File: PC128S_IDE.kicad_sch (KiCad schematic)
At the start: 15 parts, among them J1 User 2MHZ Port, J3 Conn_01x02_Male, J5 Conn_01x02_Male, P1 IDE02x20, U1 74HCT02, U2 74HCT139

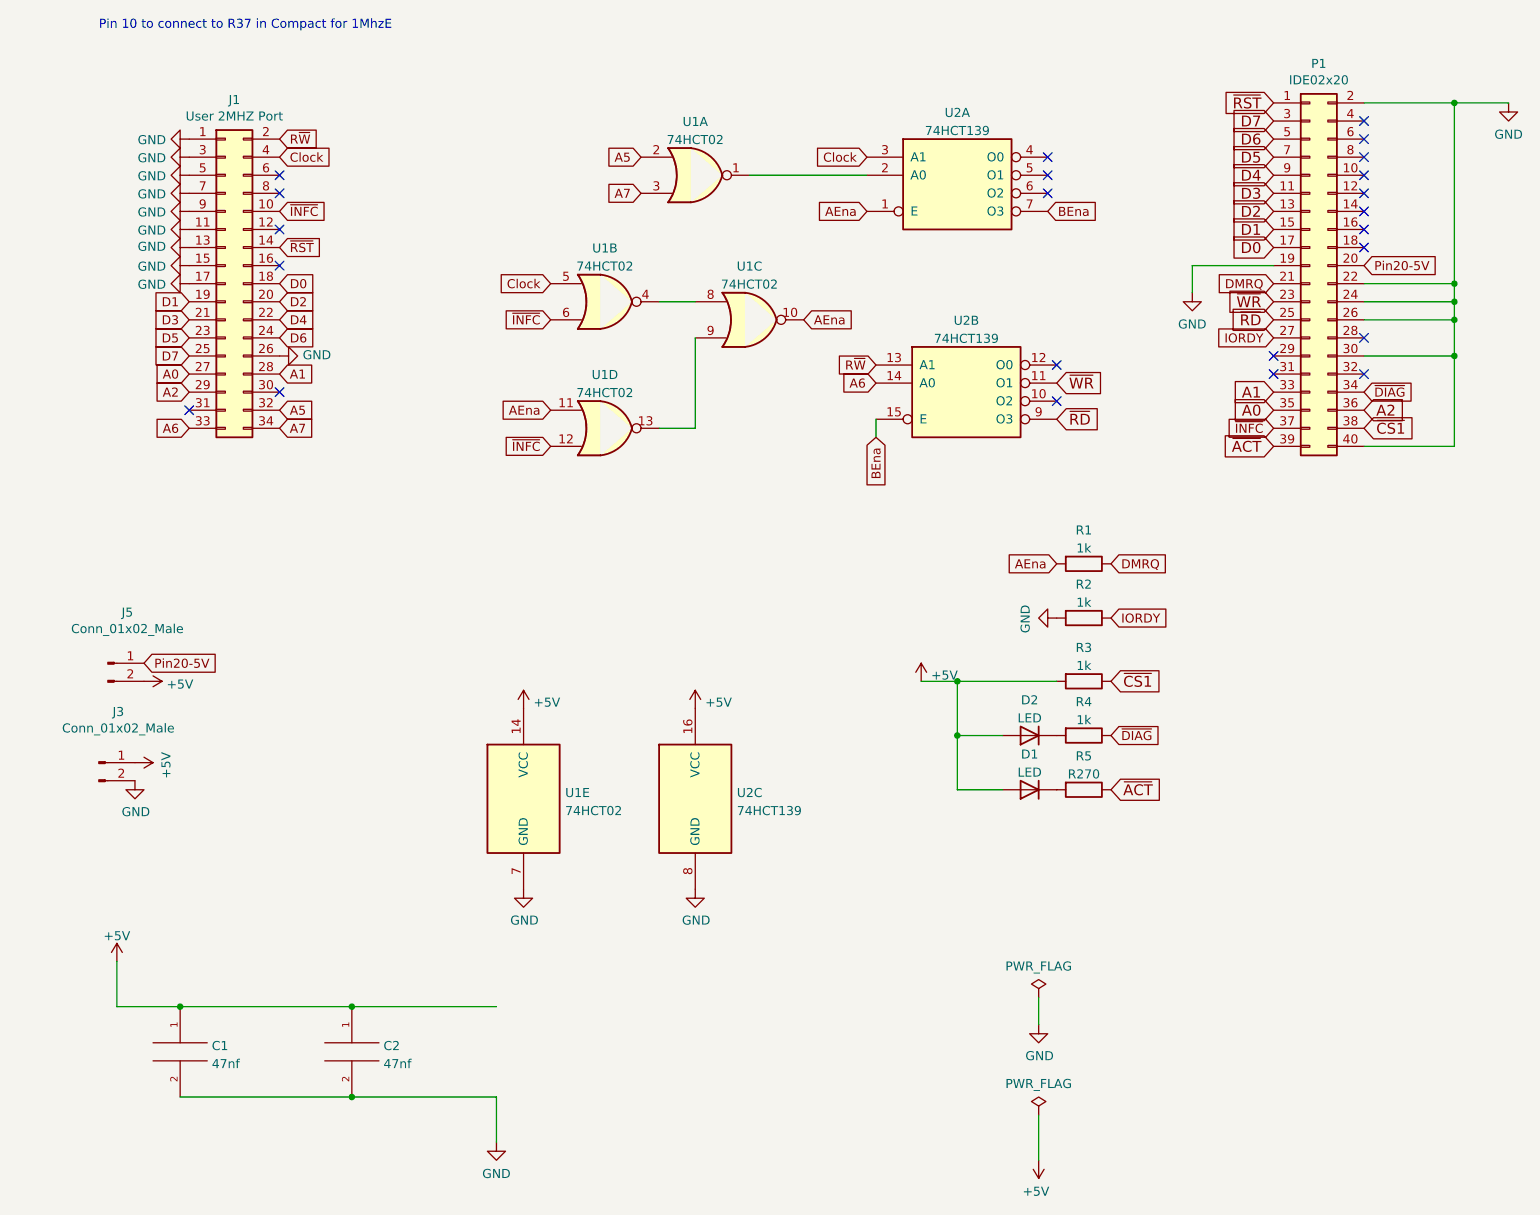
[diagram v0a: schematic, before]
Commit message: Add files via upload
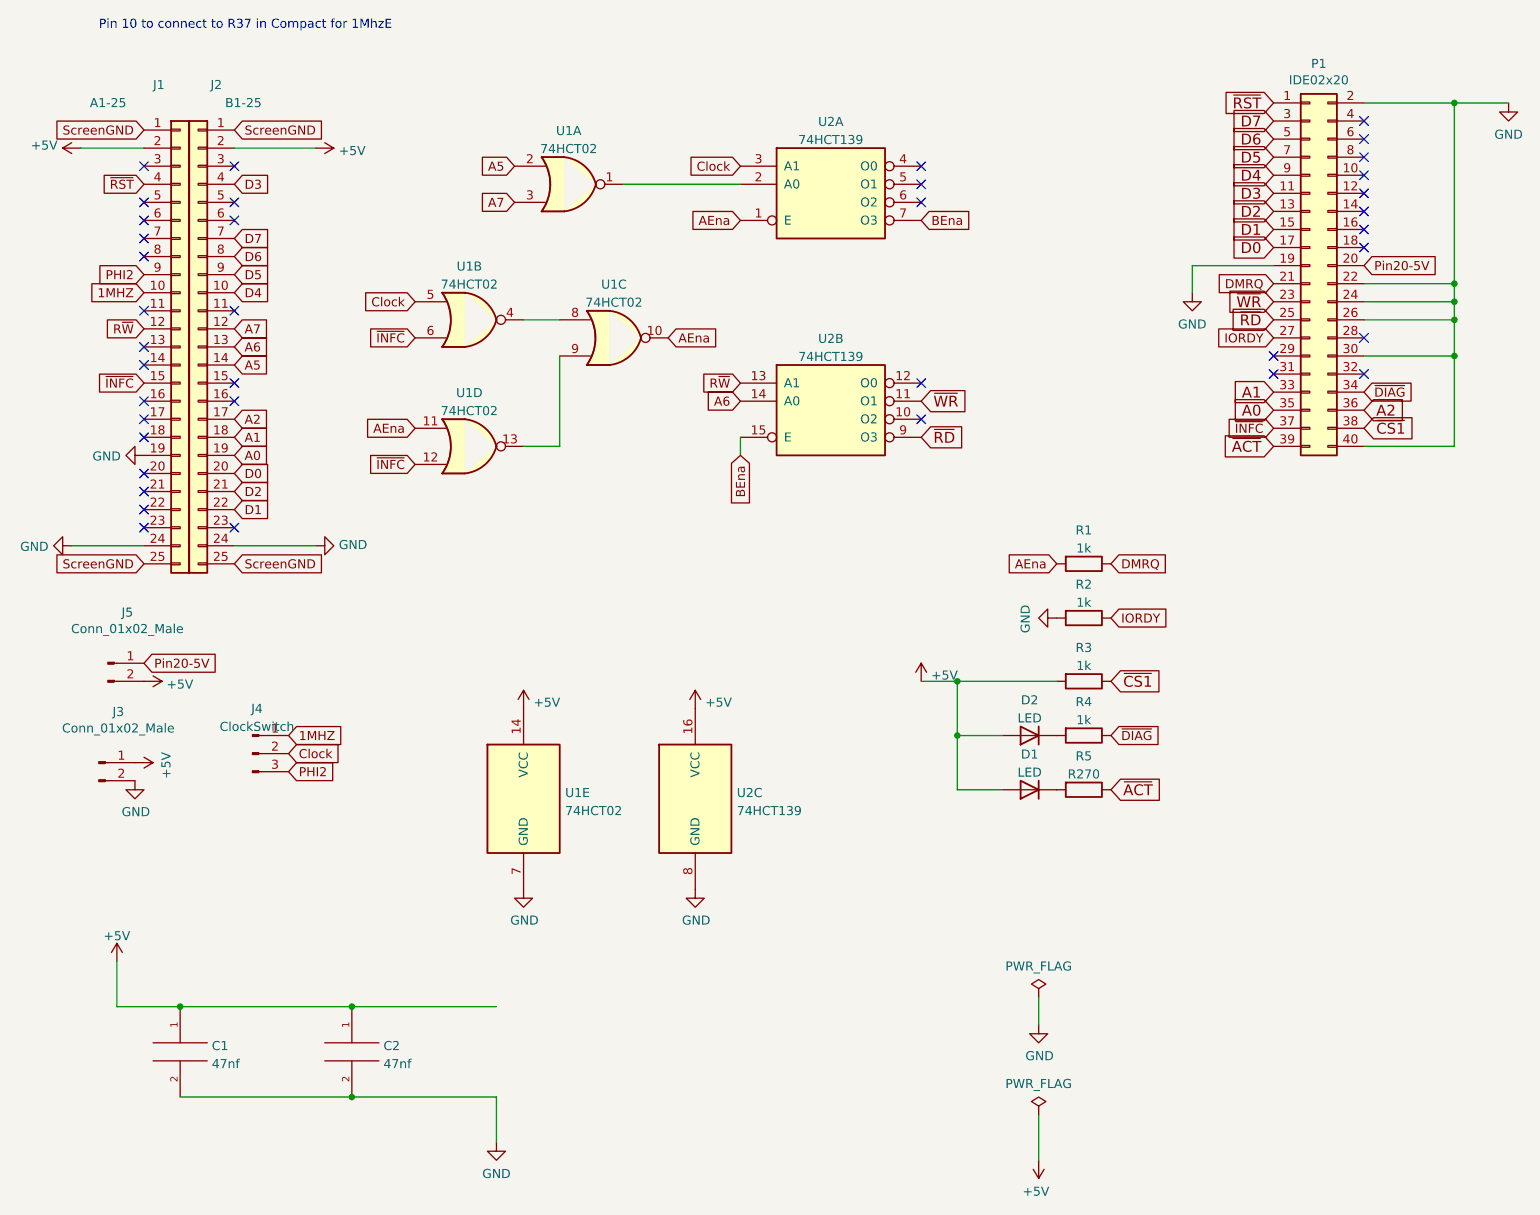
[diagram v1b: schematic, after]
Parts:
- removed J1: User 2MHZ Port, Connector_IDC:IDC-Header_2x17_P2.54mm_Vertical, symbol Connector_Generic:Conn_02x17_Odd_Even
- added J1: A1-25, Connector_PinHeader_2.54mm:PinHeader_1x25_P2.54mm_Vertical, symbol Connector_Generic:Conn_01x25
- added J2: B1-25, Connector_PinHeader_2.54mm:PinHeader_1x25_P2.54mm_Vertical, symbol Connector_Generic:Conn_01x25
- added J4: ClockSwitch, Connector_PinHeader_2.54mm:PinHeader_1x03_P2.54mm_Vertical, symbol Connector:Conn_01x03_Male
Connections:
- net +5V: now also J1.2 (Pin_2), J2.2 (Pin_2)
- net A0: now also J2.19 (Pin_19)
- net A1: now also J2.18 (Pin_18)
- net A2: now also J2.17 (Pin_17)
- net A5: now also J2.14 (Pin_14)
- net A6: now also J2.13 (Pin_13)
- net A7: now also J2.12 (Pin_12)
- net Clock: now also J4.2 (Pin_2)
- net D0: now also J2.20 (Pin_20)
- net D1: now also J2.22 (Pin_22)
- net D2: now also J2.21 (Pin_21)
- net D3: now also J2.4 (Pin_4)
- net D4: now also J2.10 (Pin_10)
- net D5: now also J2.9 (Pin_9)
- net D6: now also J2.8 (Pin_8)
- net D7: now also J2.7 (Pin_7)
- net GND: now also J1.19 (Pin_19), J1.24 (Pin_24), J2.24 (Pin_24)
- net R~{W}: now also J1.12 (Pin_12)
- net ~{INFC}: now also J1.15 (Pin_15)
- net ~{RST}: now also J1.4 (Pin_4)
- new net 1MHZ: J1.10 (Pin_10), J4.1 (Pin_1)
- new net PHI2: J1.9 (Pin_9), J4.3 (Pin_3)
- new net ScreenGND: J1.1 (Pin_1), J1.25 (Pin_25), J2.1 (Pin_1), J2.25 (Pin_25)
- no-connect marks 23 -> 39
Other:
- moved on the sheet: U1A, U1B, U1C, U1D, U2A, U2B
